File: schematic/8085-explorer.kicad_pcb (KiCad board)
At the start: 2 copper layers, 120 x 80 mm, 51 parts, among them J1 DE9_Pins_MountingHoles, J2 DC-005 Power Jack, J4 Conn_01x02_Pin, J5 Conn_01x02_Pin, J6 Conn_02x05_Odd_Even, U1 8085, U2 74LS573, U3 28C256, U4 HM62256BLP, U5 74LS14, U6 74LS32, U7 74LS74, U8 MAX232, U9 L7805, Y1 6.144 MHz

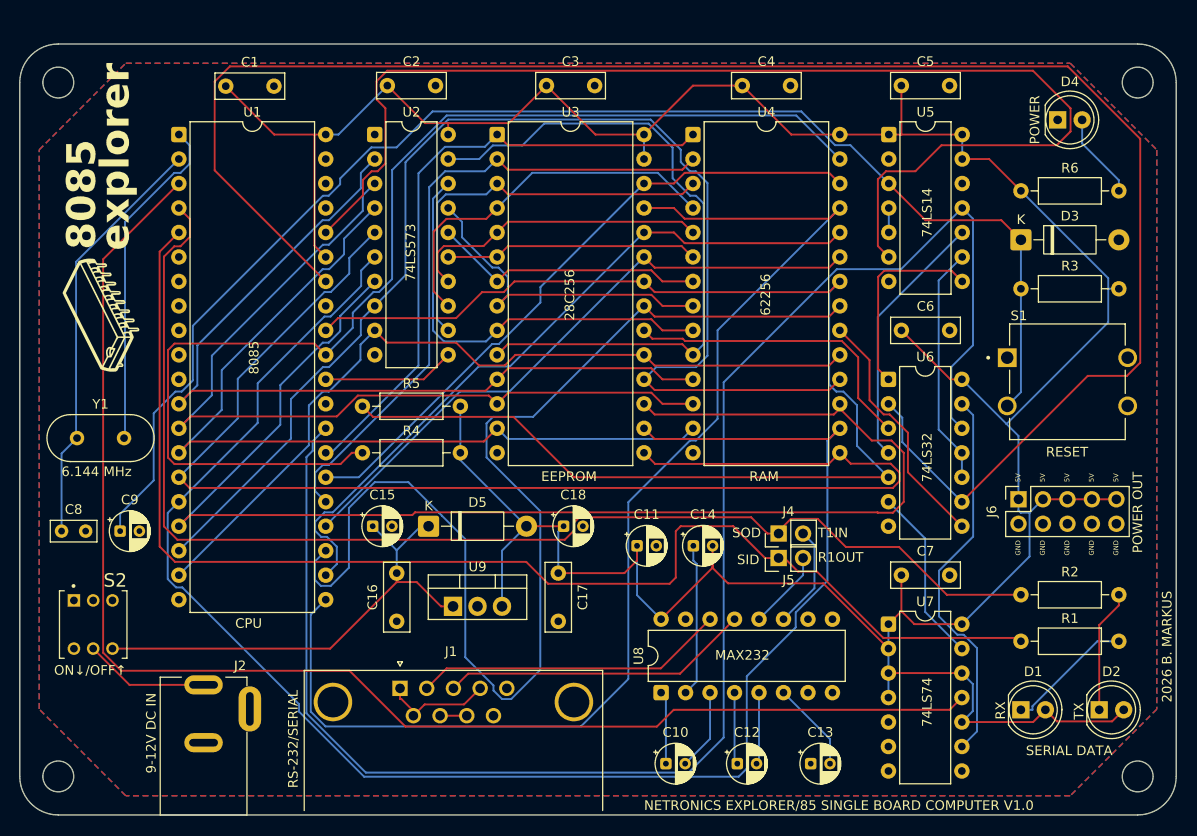
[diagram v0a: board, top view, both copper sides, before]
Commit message: PCB updated
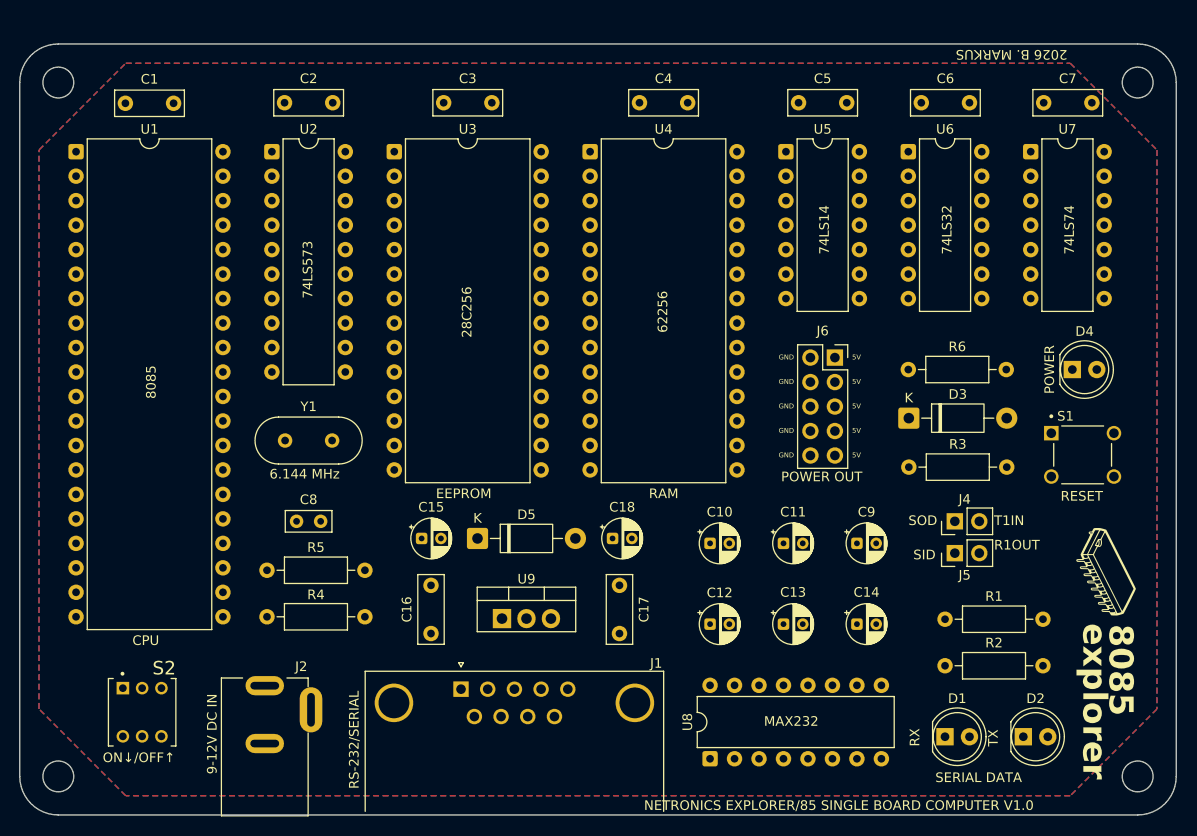
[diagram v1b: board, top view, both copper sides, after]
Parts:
- S1: value Button TACT 12x12mm -> Button TACT 6x6mm; footprint StockLib:Button TACT 12x12mm -> StockLib:Button TACT 6x6mm
- moved G1 108.3 mm to (113.0, 54.8), turned to -90 degrees
- moved C9 76.5 mm to (86.9, 51.8)
- moved C7 51.2 mm to (106.2, 6.10)
- moved U7 51.2 mm to (104.9, 11.2)
- moved D4 26.0 mm to (109.2, 33.8)
- moved C8 24.4 mm to (28.7, 49.5)
- moved J6 24.1 mm to (84.6, 32.5), turned to 0 degrees
- moved C6 23.7 mm to (93.5, 6.10)
- moved U6 23.7 mm to (92.2, 11.2)
- moved C10 23.3 mm to (71.6, 51.8)
- moved R6 21.9 mm to (92.2, 33.8)
- moved D3 21.9 mm to (92.3, 38.8)
- moved R3 21.9 mm to (92.3, 43.9)
- moved Y1 21.6 mm to (27.5, 41.1)
- moved R5 19.7 mm to (25.7, 54.6)
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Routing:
- net +5V: track 342.1 -> 0.00 mm
- net IO_~{M}: track 186.3 -> 0.00 mm
- net /D4: track 172.6 -> 0.00 mm
- net A15: track 171.6 -> 0.00 mm
- net /D5: track 145.6 -> 0.00 mm
- net RESET_OUT: track 145.5 -> 0.00 mm
- net Net-(D3-K): track 143.6 -> 0.00 mm
- net /D3: track 138.9 -> 0.00 mm
- net ~{RD}: track 137.8 -> 0.00 mm
- net UART_RX: track 134.6 -> 0.00 mm
- net /D6: track 133.8 -> 0.00 mm
- net UART_TX: track 130.7 -> 0.00 mm
- net /A8: track 127.5 -> 0.00 mm
- net Net-(U1-~{RESET_IN}): track 126.0 -> 0.00 mm
- net /A10: track 123.8 -> 0.00 mm
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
